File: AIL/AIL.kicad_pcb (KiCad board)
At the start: 2 copper layers, 106 x 48.6 mm, 36 parts, among them J1 Screw_Terminal_01x02, J2 Screw_Terminal_01x02, Q1 BC548, U1 TPL290

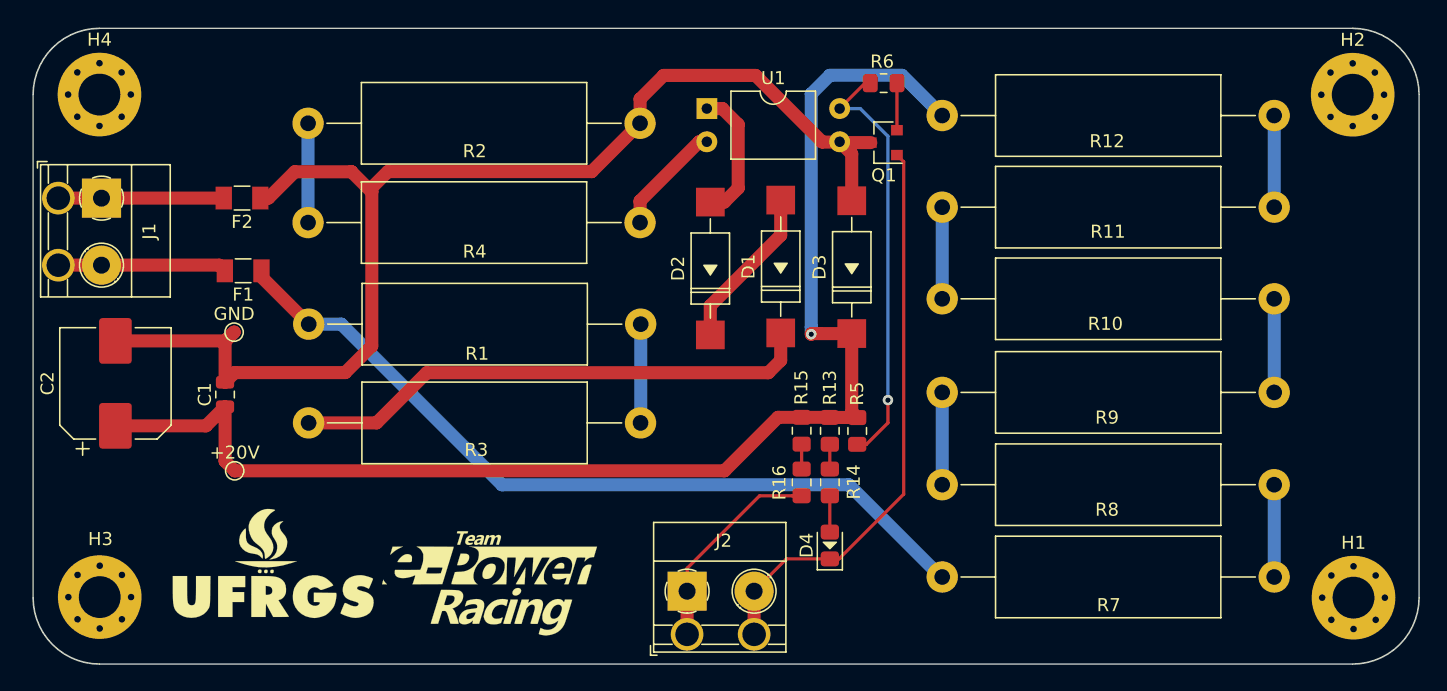
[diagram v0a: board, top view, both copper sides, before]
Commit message: geretate BSPD gerbers
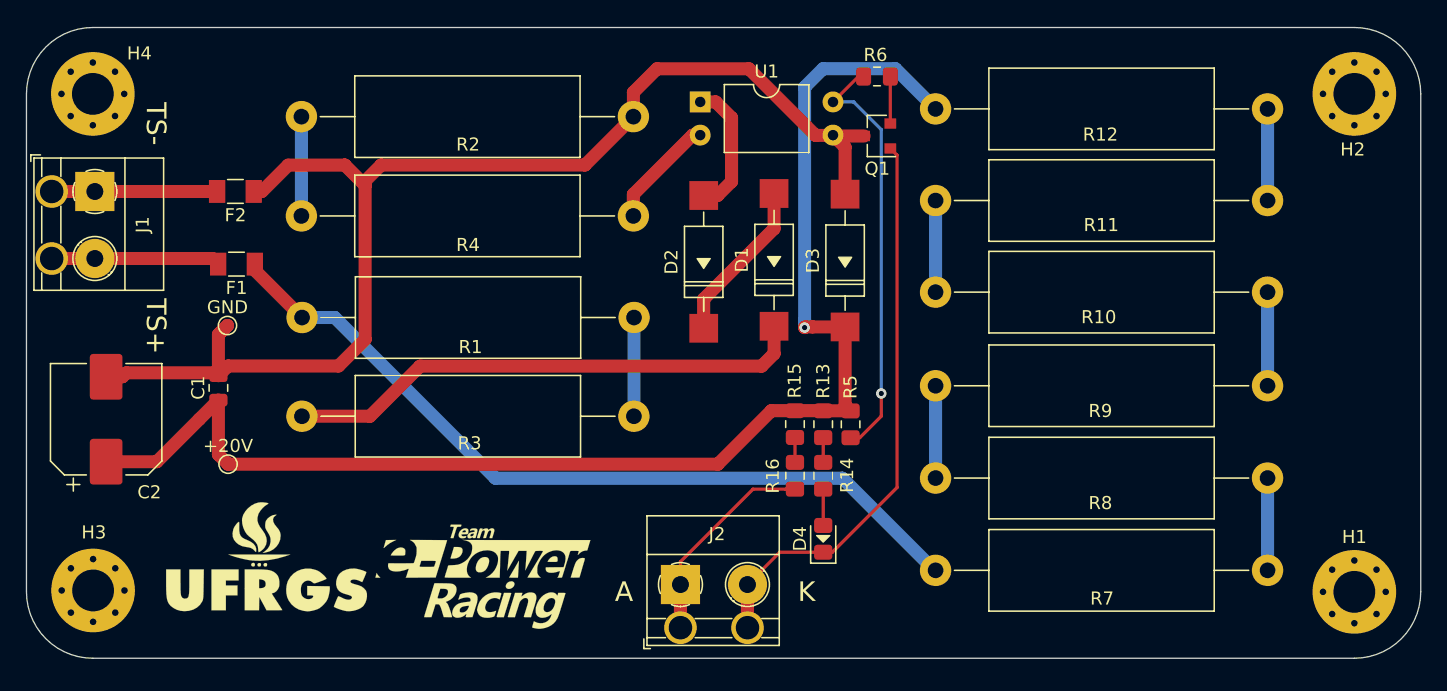
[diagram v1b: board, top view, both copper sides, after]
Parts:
- moved C2 2.83 mm to (72.1, 116.3)
- moved D3 0.72 mm to (128.7, 109.3)
- moved F2 0.72 mm to (82.0, 98.9)
- moved R11 0.72 mm to (161.0, 99.6)
- moved R15 0.72 mm to (124.8, 116.7)
- moved R3 0.72 mm to (87.1, 116.1)
- moved R5 0.72 mm to (129.1, 116.7)
- moved R6 0.72 mm to (131.1, 90.1)
- moved R7 0.72 mm to (161.0, 127.9)
- moved TP1 0.72 mm to (81.5, 119.8)
- moved D1 0.72 mm to (123.2, 109.2)
- moved D2 0.72 mm to (117.9, 109.4)
- moved F1 0.72 mm to (82.1, 104.5)
- moved G1 0.72 mm to (100.9, 128.4)
- moved G2 0.72 mm to (84.4, 126.8)
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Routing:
- net +20V: track 103.5 -> 105.1 mm
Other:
- board size 106 x 48.6 mm -> 106.7 x 48.3 mm
- board text added: "> AIL"
- board text added: "> Leonardo Motta"
- board text added: "> Rev. A | 18.09.2020"
- board text added: "> e-Power UFRGS"
- board text added: "A"
- board text added: "K"
- board text added: "TESTED"
- board text added: "TS+"
- board text added: "TS-"
